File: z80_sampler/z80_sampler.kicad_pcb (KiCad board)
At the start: 2 copper layers, 71.1 x 53.3 mm, 21 parts, among them U2 74HCT574, U3 74HCT10, U4 74HC86, U6 74HCT574, U7 74HCT245

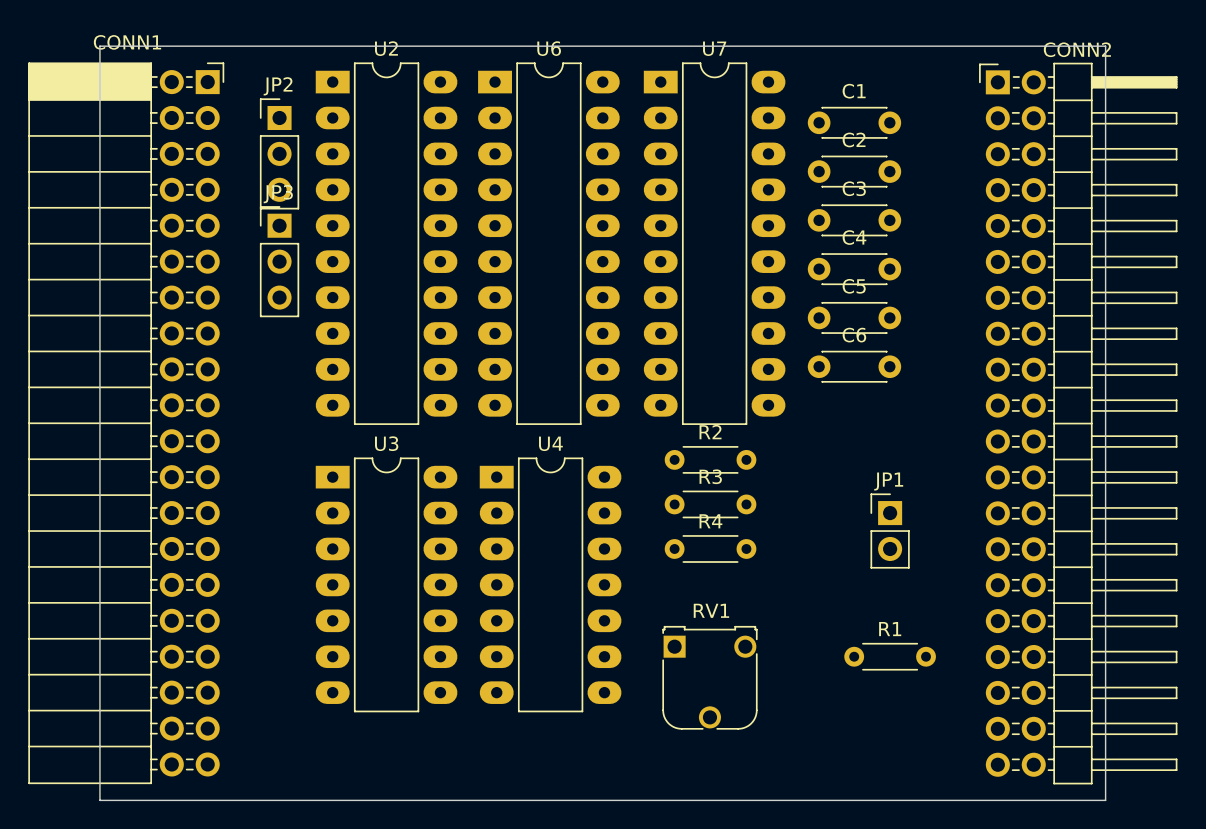
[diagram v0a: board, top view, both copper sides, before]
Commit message: Z80 sampler project complete.
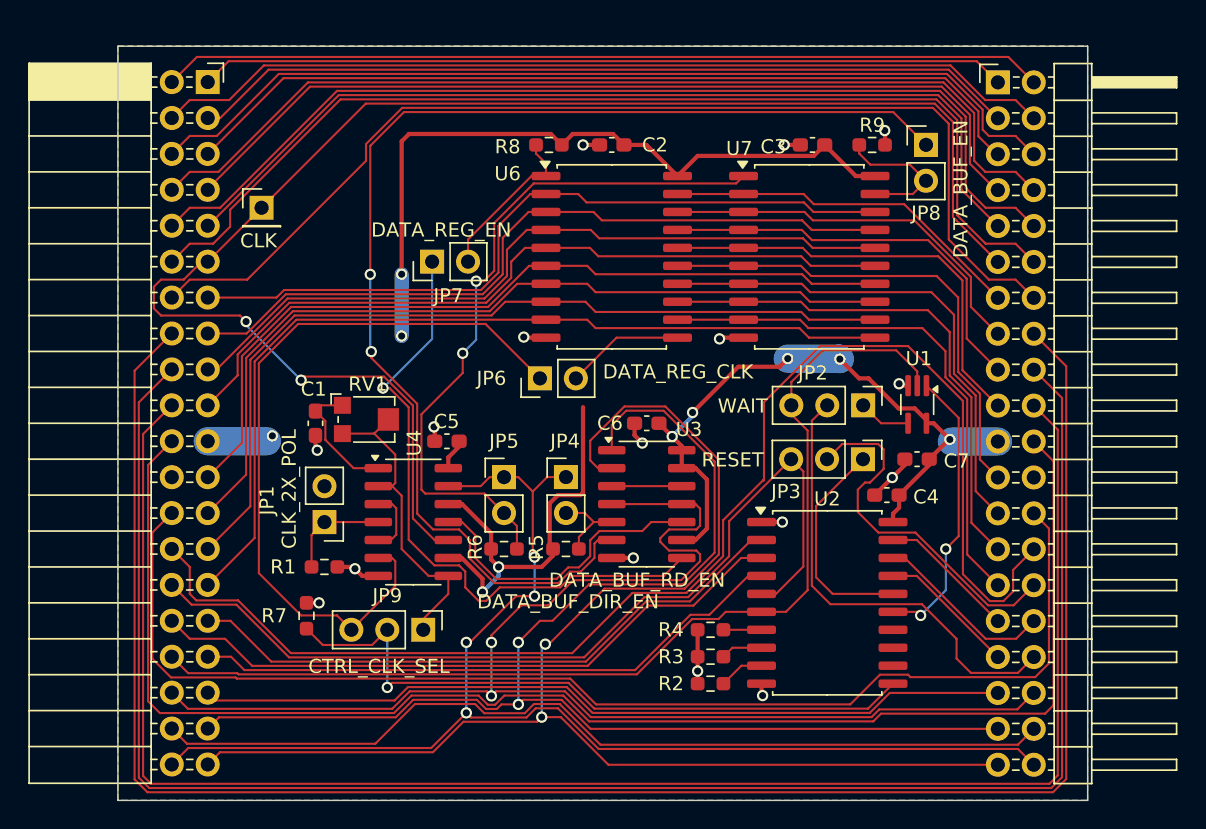
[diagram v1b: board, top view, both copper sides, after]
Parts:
- added C7: 1u, Capacitor_SMD:C_0603_1608Metric_Pad1.08x0.95mm_HandSolder, F.Cu at (95.9, 47.0)
- added JP4: Jumper_2_Bridged, Connector_PinHeader_2.54mm:PinHeader_1x02_P2.54mm_Vertical, F.Cu at (71.1, 48.3)
- added JP5: Jumper_2_Open, Connector_PinHeader_2.54mm:PinHeader_1x02_P2.54mm_Vertical, F.Cu at (66.7, 48.3)
- added JP6: Jumper_2_Bridged, Connector_PinHeader_2.54mm:PinHeader_1x02_P2.54mm_Vertical, F.Cu at (69.2, 41.3)
- added JP7: Jumper_2_Bridged, Connector_PinHeader_2.54mm:PinHeader_1x02_P2.54mm_Vertical, F.Cu at (61.6, 33.0)
- added JP8: Jumper_2_Bridged, Connector_PinHeader_2.54mm:PinHeader_1x02_P2.54mm_Vertical, F.Cu at (96.5, 24.8)
- added JP9: Jumper_3_Bridged12, Connector_PinHeader_2.54mm:PinHeader_1x03_P2.54mm_Vertical, F.Cu at (61.0, 59.1)
- added R5: 10k, Resistor_SMD:R_0603_1608Metric_Pad0.98x0.95mm_HandSolder, F.Cu at (71.1, 53.3)
- added R6: 10k, Resistor_SMD:R_0603_1608Metric_Pad0.98x0.95mm_HandSolder, F.Cu at (66.7, 53.3)
- added R7: 10k, Resistor_SMD:R_0603_1608Metric_Pad0.98x0.95mm_HandSolder, F.Cu at (52.7, 58.1)
- added R8: 10k, Resistor_SMD:R_0603_1608Metric_Pad0.98x0.95mm_HandSolder, F.Cu at (69.8, 24.8)
- added R9: 10k, Resistor_SMD:R_0603_1608Metric_Pad0.98x0.95mm_HandSolder, F.Cu at (92.7, 24.8)
- added TP1: TestPoint, Connector_PinHeader_2.54mm:PinHeader_1x01_P2.54mm_Vertical, F.Cu at (49.5, 29.2)
- added U1: 74AHCT1G08, Package_TO_SOT_SMD:SOT-353_SC-70-5_Handsoldering, F.Cu at (95.9, 43.1)
- C1, C2, C3, C4, C5, C6: footprint Capacitor_THT:C_Disc_D4.3mm_W1.9mm_P5.00mm -> Capacitor_SMD:C_0603_1608Metric_Pad1.08x0.95mm_HandSolder
- R1, R2, R3, R4: footprint Resistor_THT:R_Axial_DIN0204_L3.6mm_D1.6mm_P5.08mm_Horizontal -> Resistor_SMD:R_0603_1608Metric_Pad0.98x0.95mm_HandSolder
- RV1: footprint Potentiometer_THT:Potentiometer_Runtron_RM-065_Vertical -> Potentiometer_SMD:Potentiometer_Bourns_TC33X_Vertical
- U2, U6: footprint Package_DIP:DIP-20_W7.62mm_LongPads -> Package_SO:SOIC-20W_7.5x12.8mm_P1.27mm
- U3, U4: footprint Package_DIP:DIP-14_W7.62mm_LongPads -> Package_SO:SOIC-14_3.9x8.7mm_P1.27mm
- U7: value 74HCT245 -> SN74CBT3245CDW; footprint Package_DIP:DIP-20_W7.62mm_LongPads -> Package_SO:SOIC-20W_7.5x12.8mm_P1.27mm
- moved U2 50.8 mm to (89.5, 57.1)
- moved JP2 46.0 mm to (92.1, 43.2), turned to -90 degrees
- moved JP3 44.4 mm to (92.1, 47.0), turned to -90 degrees
- moved C1 41.5 mm to (53.3, 44.5), turned to -90 degrees
- moved JP1 40.0 mm to (54.0, 51.4), turned to 180 degrees
- moved R1 38.0 mm to (54.0, 54.6)
- moved C5 27.7 mm to (62.6, 45.7), turned to 180 degrees
- moved RV1 27.0 mm to (57.0, 44.2)
- moved U3 22.3 mm to (76.8, 50.2)
- moved C4 16.7 mm to (93.8, 49.5), turned to 180 degrees
- moved U7 16.2 mm to (88.3, 32.7)
- moved R2 16.0 mm to (81.3, 62.9), turned to 180 degrees
- moved U6 14.9 mm to (74.3, 32.7)
- moved C2 14.8 mm to (74.3, 24.8), turned to 180 degrees
- moved C6 12.8 mm to (76.8, 44.5), turned to 180 degrees
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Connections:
- JP2 pad 1: /HOST_WAIT_N -> Net-(JP2-A)
- JP2 pad 3: Net-(JP2-B) -> /HOST_WAIT_N
- U2 pad 11: /CLK_N -> Net-(JP9-C)
- U2 pad 15: Net-(JP2-B) -> Net-(U2-Q4)
- U2 pad 17: /BUSREQ_N -> /NMI_N
- U2 pad 18: /INT_N -> /BUSREQ_N
- U2 pad 19: /NMI_N -> /INT_N
- U2 pad 2: /HOST_NMI_N -> /HOST_INT_N
- U2 pad 3: /HOST_INT_N -> /HOST_BUSREQ_N
- U2 pad 4: /HOST_BUSREQ_N -> /HOST_NMI_N
- U3 pad 5: /RN_N -> Net-(JP4-B)
- U3 pad 6: Net-(U7-CE) -> Net-(JP8-A)
- U3 pad 8: Net-(U6-OE) -> Net-(JP7-A)
- U4 pad 13: /RN_N -> /RD_N
- U6 pad 1: Net-(U6-OE) -> Net-(JP7-B)
- U6 pad 11: /CLK_2X -> Net-(JP6-B)
- U7 pad 1: GND -> Net-(JP5-B)
- U7 pad 11: /D1 -> /HOST_D1
- U7 pad 12: /D0 -> /HOST_D0
- U7 pad 13: /D7 -> /HOST_D7
- U7 pad 14: /D2 -> /HOST_D2
- U7 pad 15: /D6 -> /HOST_D6
- U7 pad 16: /D5 -> /HOST_D5
- U7 pad 17: /D3 -> /HOST_D3
- U7 pad 18: /D4 -> /HOST_D4
- U7 pad 19: Net-(U7-CE) -> Net-(JP8-B)
- U7 pad 2: /HOST_D4 -> /D4
- U7 pad 3: /HOST_D3 -> /D3
- U7 pad 4: /HOST_D5 -> /D5
- U7 pad 5: /HOST_D6 -> /D6
- U7 pad 6: /HOST_D2 -> /D2
- U7 pad 7: /HOST_D7 -> /D7
- U7 pad 8: /HOST_D0 -> /D0
- U7 pad 9: /HOST_D1 -> /D1
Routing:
- net VCC: track 0.00 -> 135.2 mm, vias 0 -> 10
- net /A3: track 0.00 -> 131.7 mm
- net /A2: track 0.00 -> 125.4 mm
- net /A1: track 0.00 -> 119.1 mm
- net /CLK: track 0.00 -> 107.8 mm, vias 0 -> 2
- net /A0: track 0.00 -> 105.0 mm
- net /IORQ_N: track 0.00 -> 100.3 mm, vias 0 -> 2
- net /BUSAK_N: track 0.00 -> 99.6 mm, vias 0 -> 2
- net /MREQ_N: track 0.00 -> 96.4 mm, vias 0 -> 2
- net /M1_N: track 0.00 -> 95.9 mm
- net /RD_N: track 0.00 -> 92.6 mm, vias 0 -> 4
- net /REFSH_N: track 0.00 -> 88.0 mm
- net Net-(JP8-A): track 0.00 -> 87.1 mm, vias 0 -> 2
- net /A4: track 0.00 -> 77.6 mm
- net /A5: track 0.00 -> 75.1 mm
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- added copper zone on B.Cu, net GND
- added copper zone on F.Cu, net VCC
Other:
- board size 71.1 x 53.3 mm -> 68.6 x 53.3 mm
- board text added: "CLK"
- board text added: "CLK_2X_POL"
- board text added: "CTRL_CLK_SEL"
- board text added: "DATA_BUF_DIR_EN"
- board text added: "DATA_BUF_EN"
- board text added: "DATA_BUF_RD_EN"
- board text added: "DATA_REG_CLK"
- board text added: "DATA_REG_EN"
- board text added: "RESET"
- board text added: "WAIT"
